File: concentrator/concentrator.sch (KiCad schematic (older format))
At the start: 20 parts, among them Q1 BS170, Q2 BS170, Q3 BS170, Q4 BS170

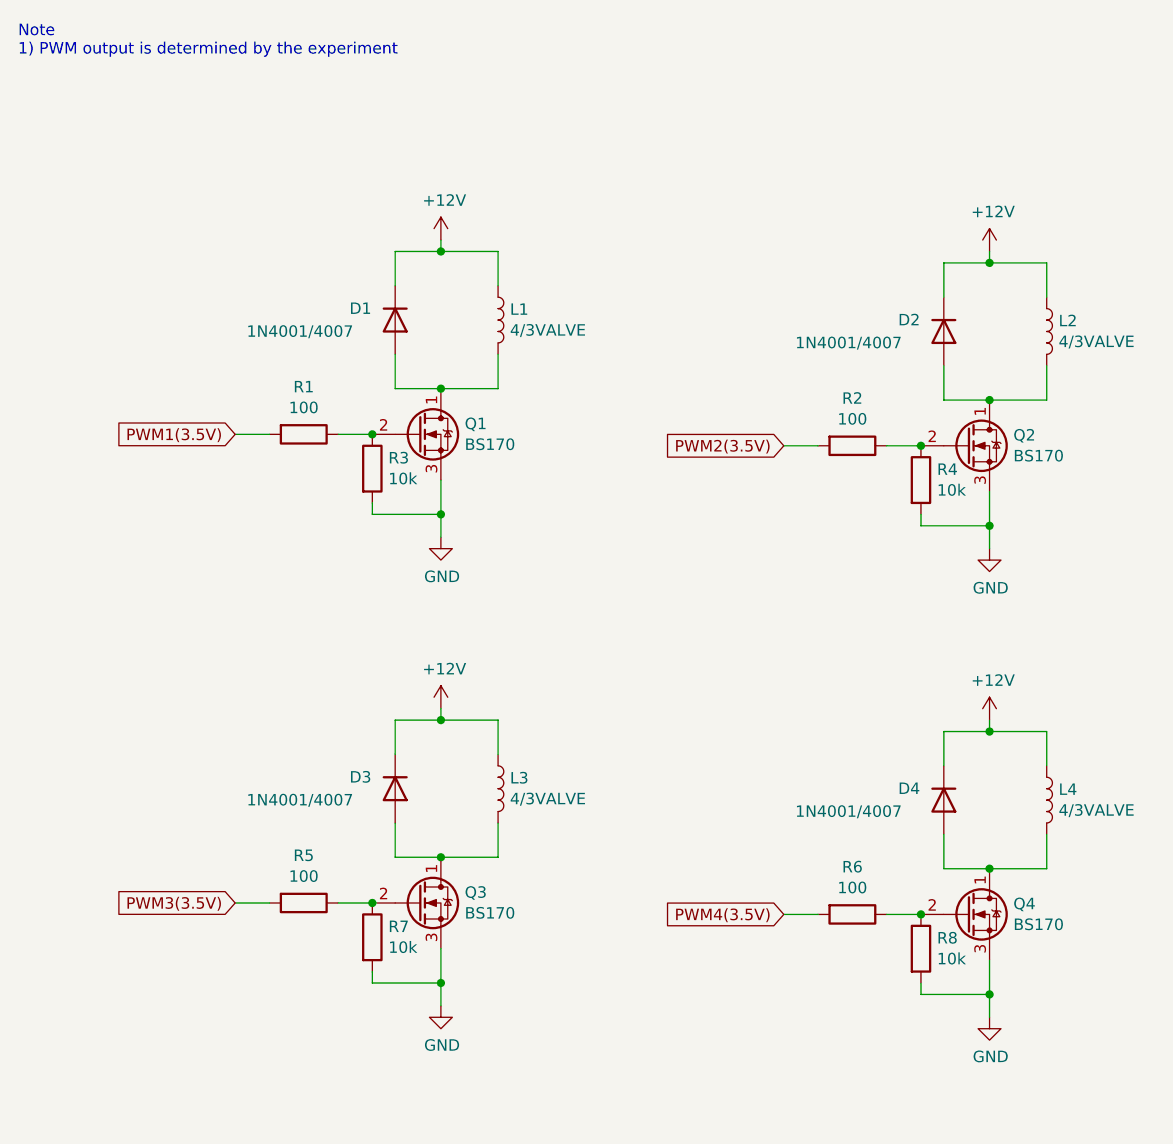
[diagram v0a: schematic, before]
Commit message: update
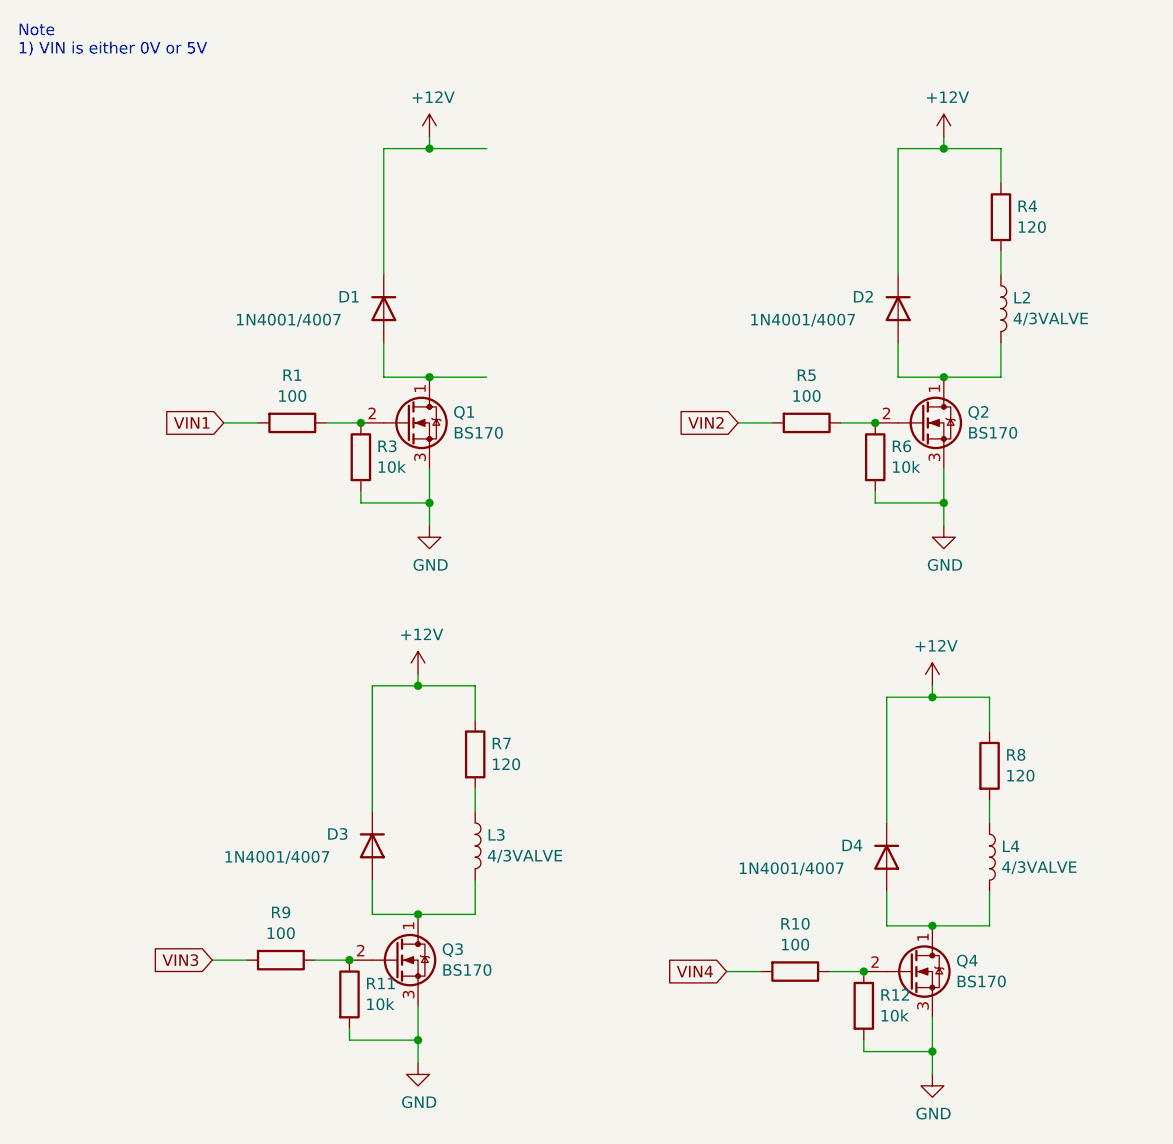
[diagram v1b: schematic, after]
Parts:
- removed L1: 4/3VALVE, symbol Device:L
- removed R2: 100, symbol Device:R
- added R10, R9: 100, symbol Device:R
- added R11, R12: 10k, symbol Device:R
- R4, R7, R8: value 10k -> 120
- R6: value 100 -> 10k
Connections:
- net labels added: VIN1, VIN2, VIN3, VIN4
- net labels removed: PWM1(3.5V), PWM2(3.5V), PWM3(3.5V), PWM4(3.5V)
- wire segments 60 -> 61
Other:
- note added: "Note\n1) VIN is either 0V or 5V"
- note removed: "Note\n1) PWM output is determined by the experiment"
- moved on the sheet: D1, Q1, R1, R3
